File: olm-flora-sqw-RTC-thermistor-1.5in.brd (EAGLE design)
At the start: 37.3 x 50.8 mm, 33 parts, among them IC1 ATMEGA32U4-AU, IC2 DS3231SN, IC3 MCP73831, IC4 MCP1700-33, J1 AYZ0202, X1 USBSMD, X3 8MHz

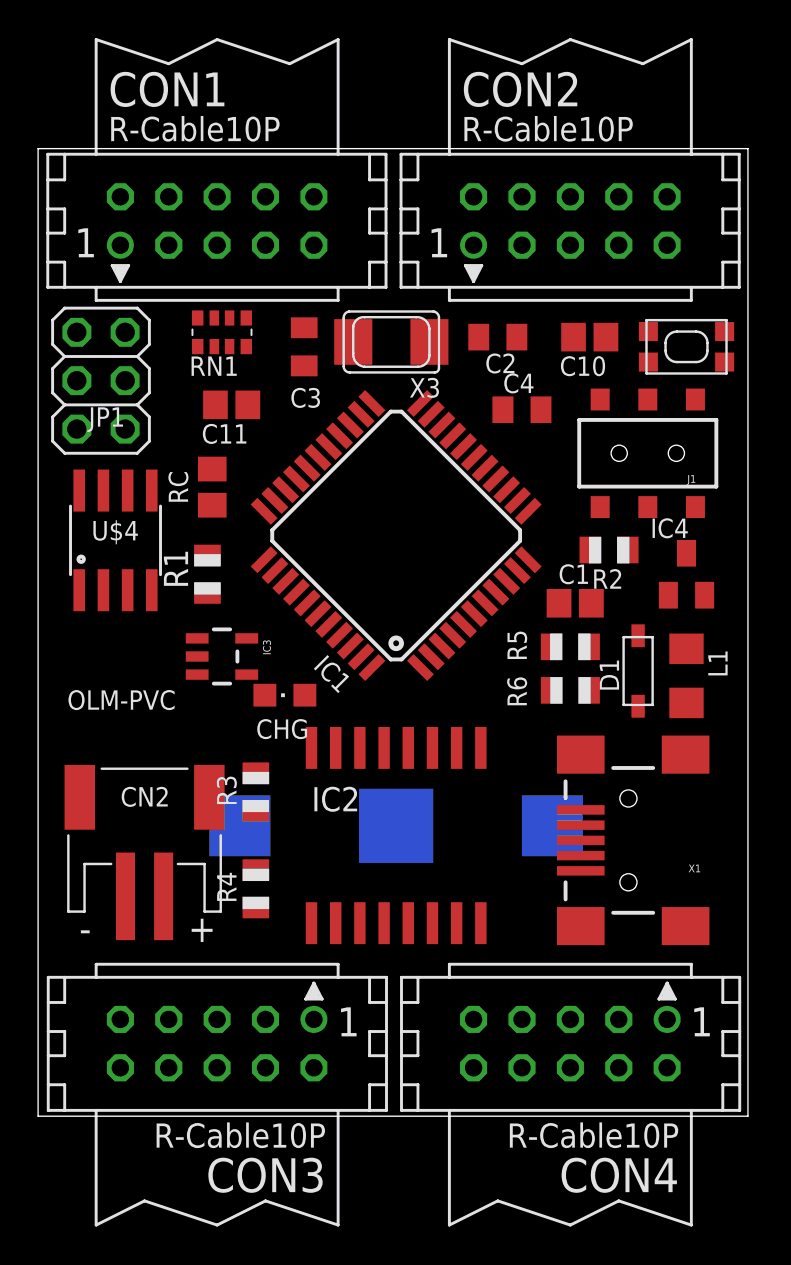
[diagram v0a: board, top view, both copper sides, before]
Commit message: update
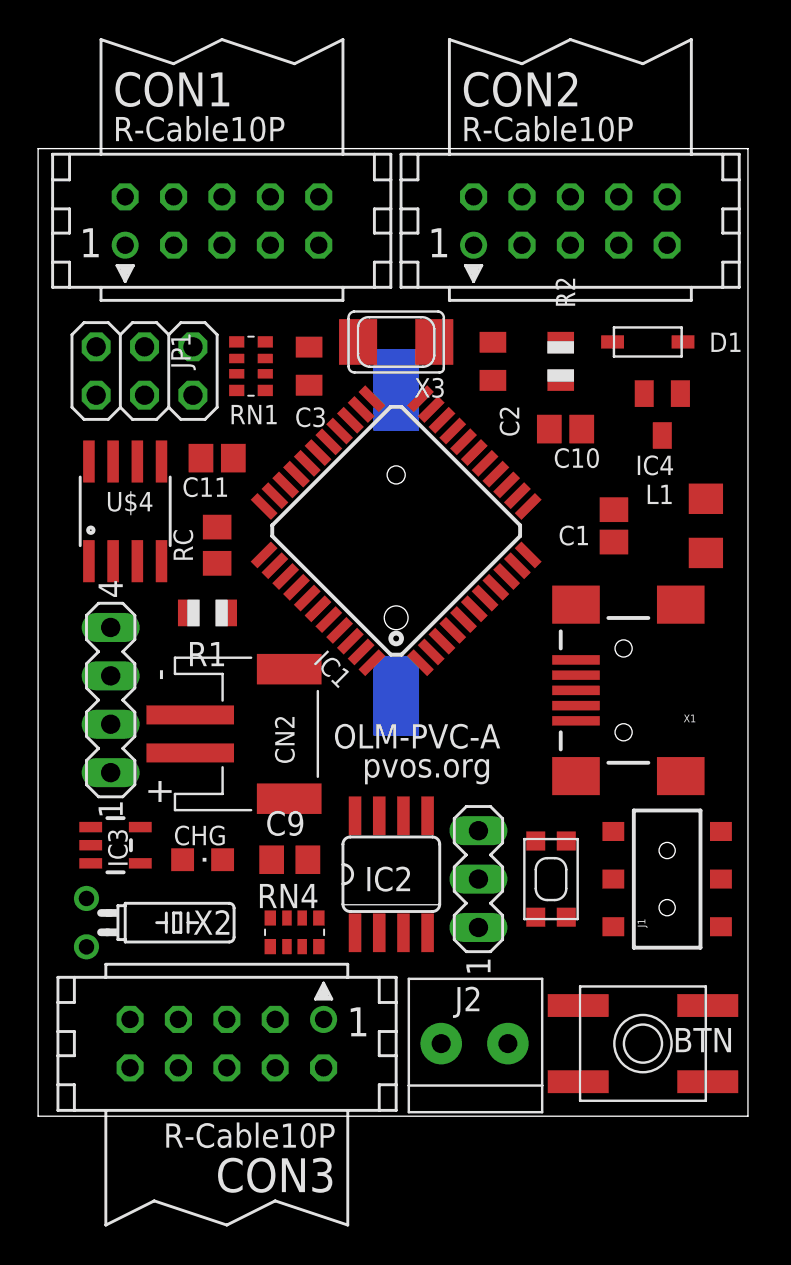
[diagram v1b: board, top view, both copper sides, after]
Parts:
- removed C4: 0.1, adafruit:C0805K
- removed CON4: (no value), con-harting:CON10
- removed R3, R4, R5, R6: 10k, adafruit:R0805
- removed U$7: BAT, adafruit:CR1220-SMD
- added BAT1: (no value), SparkFunNew:BATTCON_12MM_SMT
- added BTN: (no value), adafruit:EVQ-Q2
- added C9: 0.1u, rcl:C0805
- added J2: 1X2-3.5MM, adafruit:1X2-3.5MM
- added RN4: (no value), resistor-dil:EXB38V
- added SV1: (no value), con-lstb:MA03-1
- added SV2: (no value), con-lstb:MA04-1
- added X2: 32.768kHz, crystal:TC26H
- IC2: value DS3231SN -> DS1307; device comfile:SO16W -> adafruit:SO08
- moved BOOT 28.8 mm to (26.9, 12.4), turned to 90 degrees
- moved J1 22.4 mm to (33.0, 12.4), turned to 90 degrees
- moved D1 17.3 mm to (32.0, 40.6), turned to 0 degrees
- moved IC3 11.4 mm to (4.06, 14.2)
- moved R2 10.2 mm to (27.4, 39.6), turned to 90 degrees
- moved CHG 9.66 mm to (8.64, 13.5), turned to 270 degrees
- moved IC4 8.48 mm to (32.8, 36.8), turned to 180 degrees
- moved L1 7.94 mm to (35.1, 31.0)
- moved X1 7.88 mm to (30.7, 22.4)
- moved CN2 7.78 mm to (11.7, 20.1), turned to 270 degrees
- moved C10 4.99 mm to (27.7, 36.1), turned to 0 degrees
- moved C1 4.54 mm to (30.2, 31.0), turned to 270 degrees
- moved RC 3.06 mm to (9.40, 30.0)
- moved C11 2.90 mm to (9.40, 34.5)
- moved RN1 2.34 mm to (11.2, 39.4), turned to 90 degrees
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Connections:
- removed net 32KHZ: IC2.1, R6.1
- removed net INT/SQW: IC2.3, R3.1
- new net A0: IC1.36
- new net A1: IC1.37
- new net A2: IC1.38
- new net A3: IC1.39
- new net A4: IC1.40
- new net D11: IC1.12
- new net D4: BTN.B, BTN.B', IC1.25
- new net N$30: IC2.2, X2.1
- new net N$36: BAT1.P$2, IC2.3
- new net N$6: IC2.1, X2.2
- new net VIN: C9.1, IC2.8, RN4.7, RN4.8
- net +3V3: no longer CON4.10
- net D8: now also IC1.28
- net GND: now also BAT1.P$1, BTN.A, BTN.A', C9.2, IC2.4; no longer C4.2, CON4.6, IC2.10, IC2.11, IC2.12, IC2.13, IC2.5, IC2.6, IC2.7, IC2.8, IC2.9, U$7.-
- net MISO: no longer CON4.5
- net MOSI: no longer CON4.3
- net RST: no longer IC2.4
- net SCK: no longer CON4.1
- net SCL: now also IC2.6, RN4.1; no longer IC2.16, R4.1
- net SDA: now also IC2.5, RN4.2; no longer IC2.15, R5.1
- net VBAT: no longer CON4.8, IC2.14, U$7.+$1, U$7.+$2
- net VCC: no longer C4.1, IC2.2, R3.2, R4.2, R5.2, R6.2
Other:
- board text added: "OLM-PVC-A"
- board text added: "pvos.org"
- board text removed: "OLM-PVC"
